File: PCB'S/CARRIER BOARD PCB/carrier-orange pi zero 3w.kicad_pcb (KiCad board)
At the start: 4 copper layers, 190 x 61 mm, 112 parts, among them J1 EPAPER_HAT_B, J10 USB_A - 4, J11 USB_A - 5, J12 USB_A - 6 (For Display), J13 USB_A - 7 (For RTL SDR), J14 USB_A - 2 (Extra/For phone ), J15 FAN1, J16 FAN2, J17 L-SPEAKER, J18 R-SPEAKER, J19 EXT-GPIO (BACKUP), J2 CORE1262_HF, J3 Orange Pi Zero 3W - 40-Pin GP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, J4 Conn_01x04_Pin, J5 EXT-GPIO, J6 PWR FOR DISPLAY, J7 USB_A - 1, J8 Usb-C receptable, J9 USB_A - 3, Q1 Q_PMOS_GSD, Q2 2N7002, Q3 AO3400A, Q4 AO3400A, U1 TPS54302DDCT, U2 USB2517I-JZX, U3 TPD2EUSB30DRTR, U4 L-MAX98357AETE+T, U5 R-MAX98357AETE+T, U7 MCP23017x-x-SO, Y1 24.000MHz

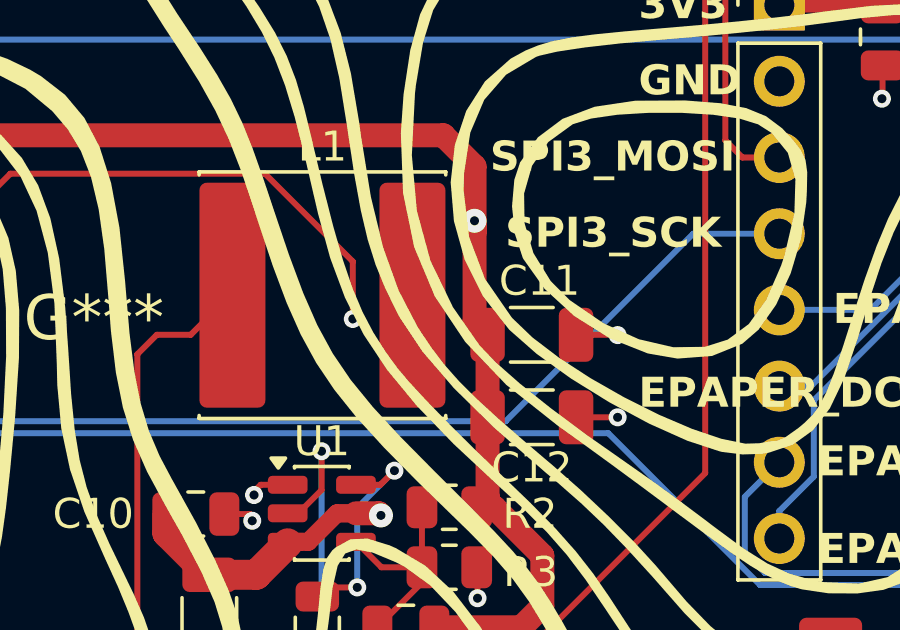
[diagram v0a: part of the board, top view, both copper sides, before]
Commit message: ain
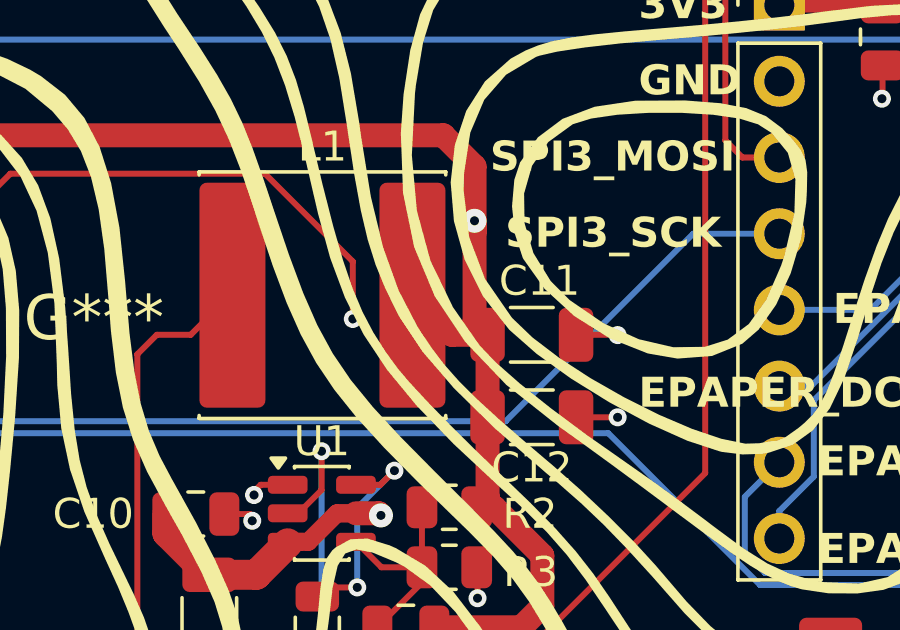
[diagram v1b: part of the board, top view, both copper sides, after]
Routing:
- net +3V3_MAIN: track 359.2 -> 362.2 mm
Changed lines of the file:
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@@
+	)
+	(segment
+		(start 141.525 62.25)
+		(end 140.34 62.25)
+		(width 0.8)
+		(layer "F.Cu")
+		(net "+3V3_MAIN")
 	)
 	(segment
@@
 		(layer "F.Cu")
 		(net "+3V3_MAIN")
+	)
+	(segment
+		(start 140.34 62.25)
+		(end 139.02 60.93)
+		(width 0.8)
+		(layer "F.Cu")
+		(net "+3V3_MAIN")
